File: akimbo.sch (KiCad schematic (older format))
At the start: 77 parts, among them J1 USB-C, J2 3.5mm TRRS, J3 3.5mm TRRS, K1 -, K11 -, K12 -, K13 -, K14 -, K15 -, K16 -, K17 -, K18 -, K19 -, K2 -, K20 -, K21 -, K22 -, K23 -, K24 -, K25 -, K26 -, K27 -, K28 -, K29 -, K3 -, K30 -, K4 -, K6 -, K7 -, K8 -, K9 -, U1 ATmega32U4, U2 MCP23017_SO, Y1 16M

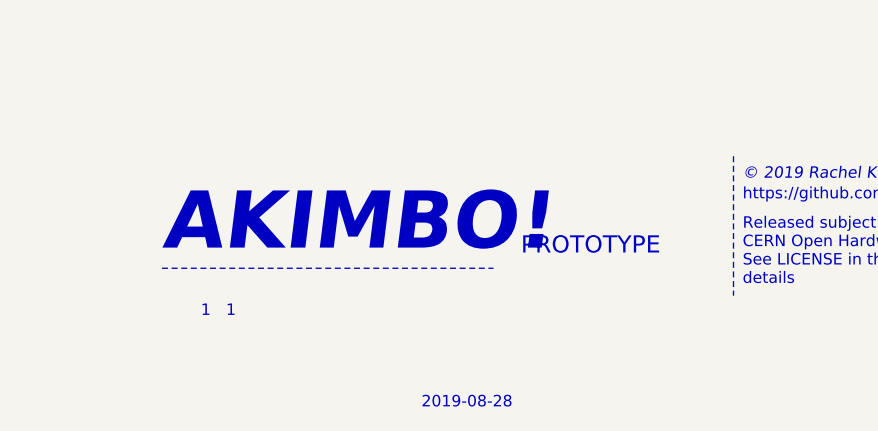
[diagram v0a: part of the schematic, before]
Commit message: minor tweaks, no functional changes
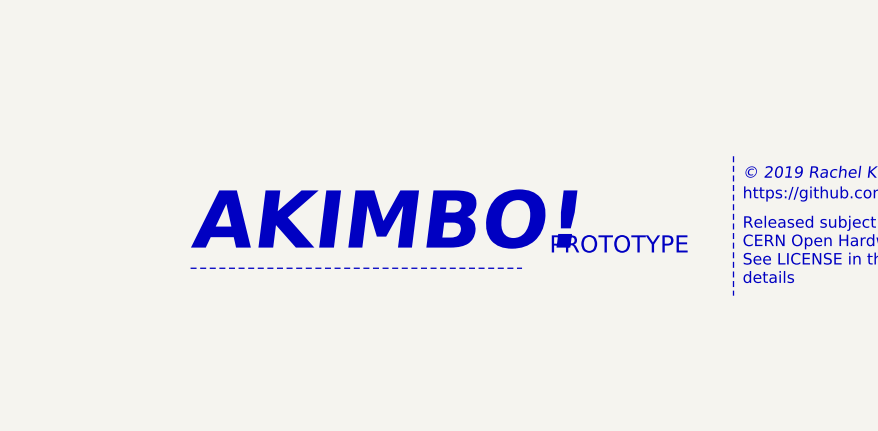
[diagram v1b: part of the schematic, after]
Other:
- note removed: "2019-08-28"
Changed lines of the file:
@@
 Wire Wire Line
 	3325 3300 3325 3200
-Text Notes 11825 10400 0    250  Italic 50
+Text Notes 11950 10400 0    250  Italic 50
 AKIMBO!
 Wire Notes Line width 48 style solid
-	11825 10450 13275 10450
-Text Notes 13395 10400 0    75   ~ 0
+	11950 10450 13400 10450
+Text Notes 13520 10400 0    75   ~ 0
 PROTOTYPE
-Text Notes 12960 11070 0    50   ~ 0
-2019-08-28
-Text Notes 11995 10670 0    50   ~ 0
-1
-Text Notes 12105 10670 0    50   ~ 0
-1
-Text Notes 14365 10070 0    50   Italic 0
-© 2019 Rachel K
-Text Notes 14365 10160 0    50   ~ 0
-https://github.com/rkanati/akimbo.git
 Wire Notes Line style solid rgb(132, 0, 0)
 	14325 9960 14325 10570
@@
 Text Notes 5500 7325 0    50   ~ 0
 Decoupling\nPlace near U1/U2 footprint
+Text Notes 14365 10160 0    50   ~ 0
+https://github.com/rkanati/akimbo.git
+Text Notes 14365 10070 0    50   Italic 0
+© 2019 Rachel K
 $EndSCHEMATC
